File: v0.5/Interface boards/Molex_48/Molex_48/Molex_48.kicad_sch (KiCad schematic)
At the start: 2 parts, among them J1 Conn_02x20_Counter_Clockwise, J2 500762-0482

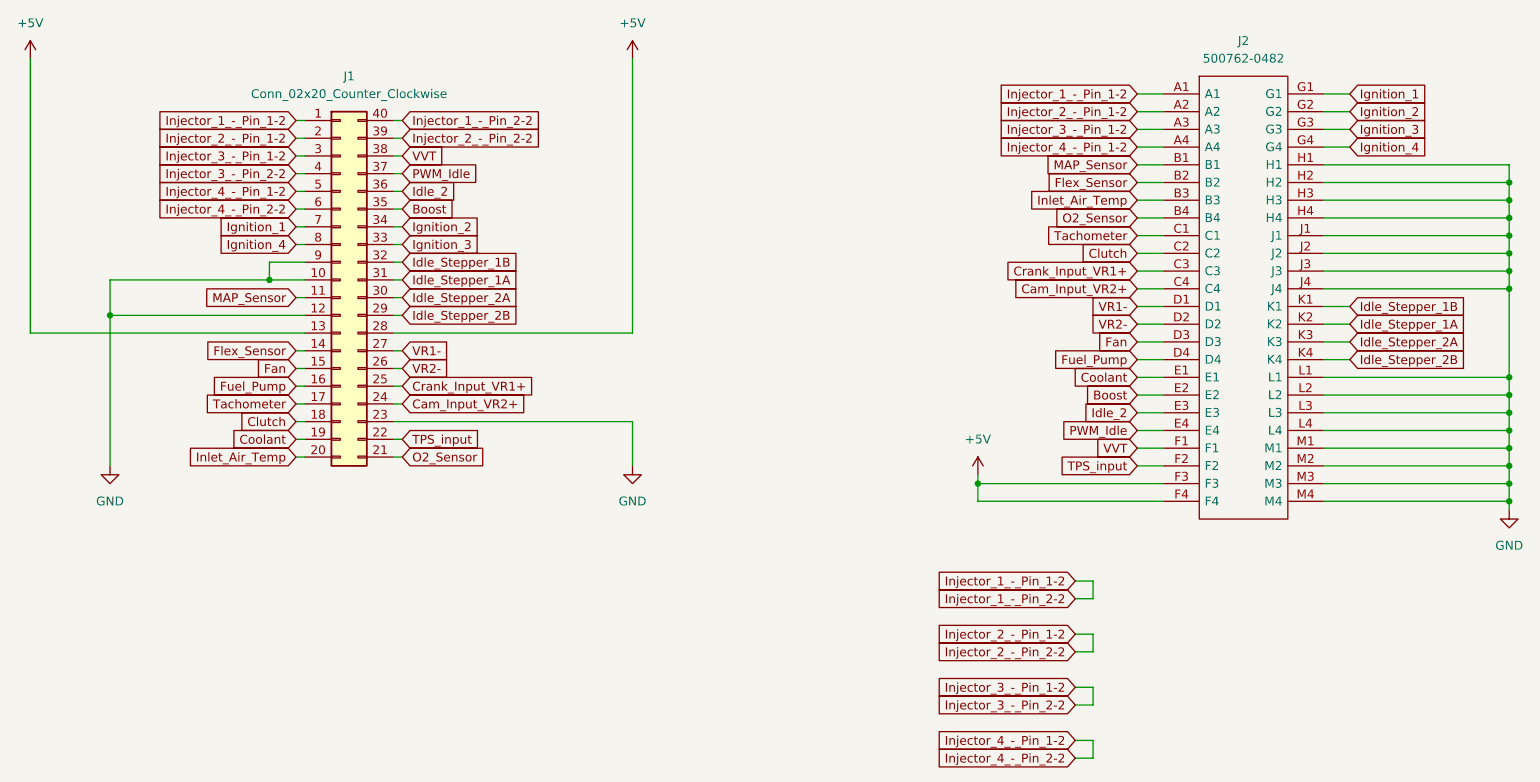
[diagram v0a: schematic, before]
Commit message: update
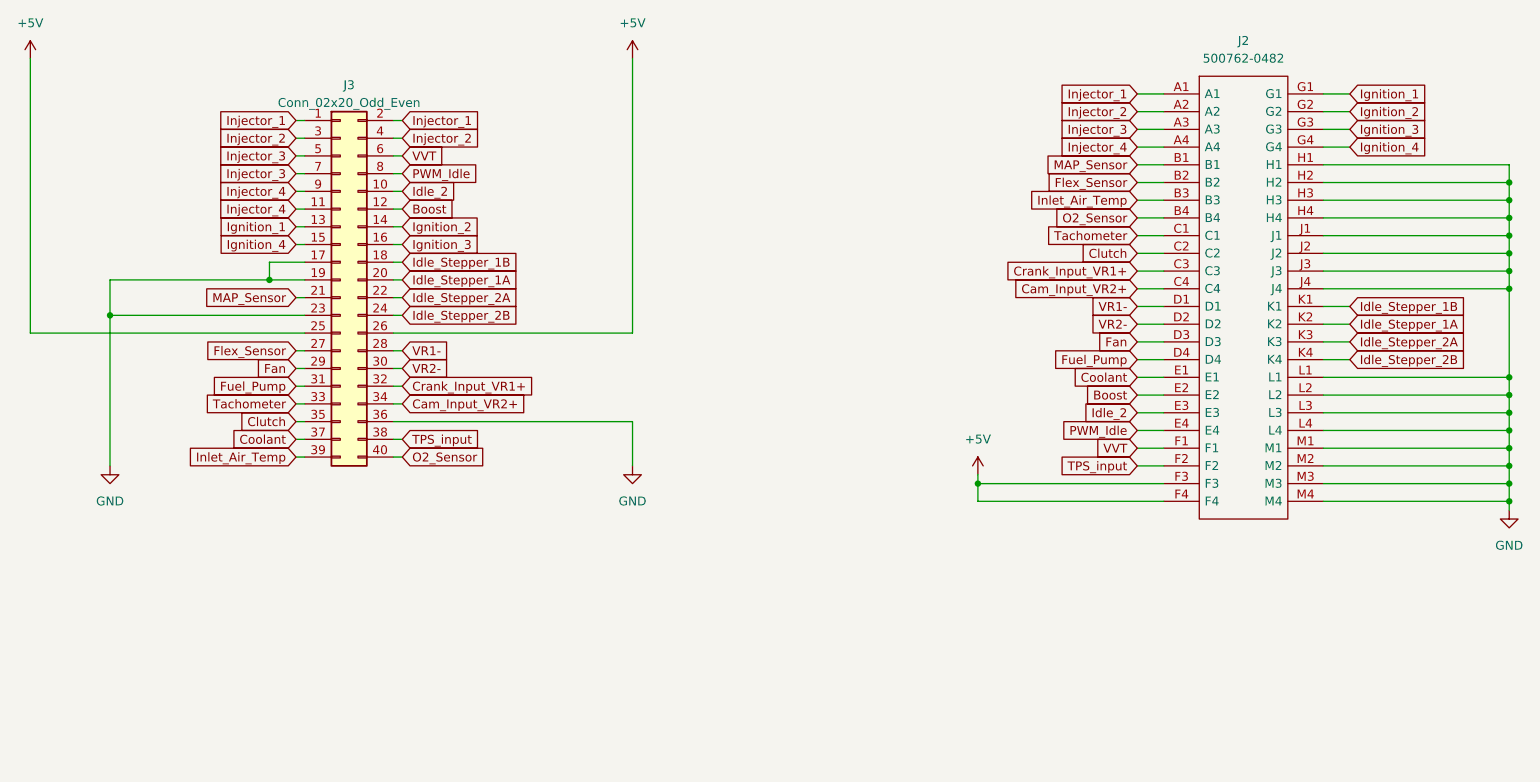
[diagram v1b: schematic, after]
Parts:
- removed J1: Conn_02x20_Counter_Clockwise, Connector_PinSocket_2.54mm:PinSocket_2x20_P2.54mm_Vertical, symbol Connector_Generic:Conn_02x20_Counter_Clockwise
- added J3: Conn_02x20_Odd_Even, Connector_PinSocket_2.54mm:PinSocket_2x20_P2.54mm_Vertical, symbol Connector_Generic:Conn_02x20_Odd_Even
- J2: footprint 5007620482 -> libs:5007620482
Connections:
- net +5V: now also J3.25 (Pin_25), J3.26 (Pin_26)
- net Boost: now also J3.12 (Pin_12)
- net Cam_Input_VR2+: now also J3.34 (Pin_34)
- net Clutch: now also J3.35 (Pin_35)
- net Coolant: now also J3.37 (Pin_37)
- net Crank_Input_VR1+: now also J3.32 (Pin_32)
- net Fan: now also J3.29 (Pin_29)
- net Flex_Sensor: now also J3.27 (Pin_27)
- net Fuel_Pump: now also J3.31 (Pin_31)
- net GND: now also J3.17 (Pin_17), J3.19 (Pin_19), J3.23 (Pin_23), J3.36 (Pin_36)
- net Idle_2: now also J3.10 (Pin_10)
- net Idle_Stepper_1A: now also J3.20 (Pin_20)
- net Idle_Stepper_1B: now also J3.18 (Pin_18)
- net Idle_Stepper_2A: now also J3.22 (Pin_22)
- net Idle_Stepper_2B: now also J3.24 (Pin_24)
- net Ignition_1: now also J3.13 (Pin_13)
- net Ignition_2: now also J3.14 (Pin_14)
- net Ignition_3: now also J3.16 (Pin_16)
- net Ignition_4: now also J3.15 (Pin_15)
- net Inlet_Air_Temp: now also J3.39 (Pin_39)
- net MAP_Sensor: now also J3.21 (Pin_21)
- net O2_Sensor: now also J3.40 (Pin_40)
- net PWM_Idle: now also J3.8 (Pin_8)
- net TPS_input: now also J3.38 (Pin_38)
- net Tachometer: now also J3.33 (Pin_33)
- net VR1-: now also J3.28 (Pin_28)
- net VR2-: now also J3.30 (Pin_30)
- net VVT: now also J3.6 (Pin_6)
- net Injector_1_-_Pin_1-2 renamed Injector_1
- net Injector_1: now also J3.1 (Pin_1), J3.2 (Pin_2)
- net Injector_2_-_Pin_1-2 renamed Injector_2
- net Injector_2: now also J3.3 (Pin_3), J3.4 (Pin_4)
- net Injector_3_-_Pin_1-2 renamed Injector_3
- net Injector_3: now also J3.5 (Pin_5), J3.7 (Pin_7)
- net Injector_4_-_Pin_1-2 renamed Injector_4
- net Injector_4: now also J3.11 (Pin_11), J3.9 (Pin_9)
